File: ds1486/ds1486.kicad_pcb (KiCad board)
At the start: 4 copper layers, 30.4 x 43.9 mm, 76 parts, among them J1 DBG, J2 DBG1-16, J3 DBG17-32, J4 DS1-16, J5 DS17-32, U1 RP2040, U2 AP2112K-3.3, U3 W25Q16JVUXIQ, U4 SN74LVC8T245, U5 SN74LVC1G00DRL, U6 YSN8010SJ, U7 SN74LVC1G00DRL, Y2 E3SB12E00004EE

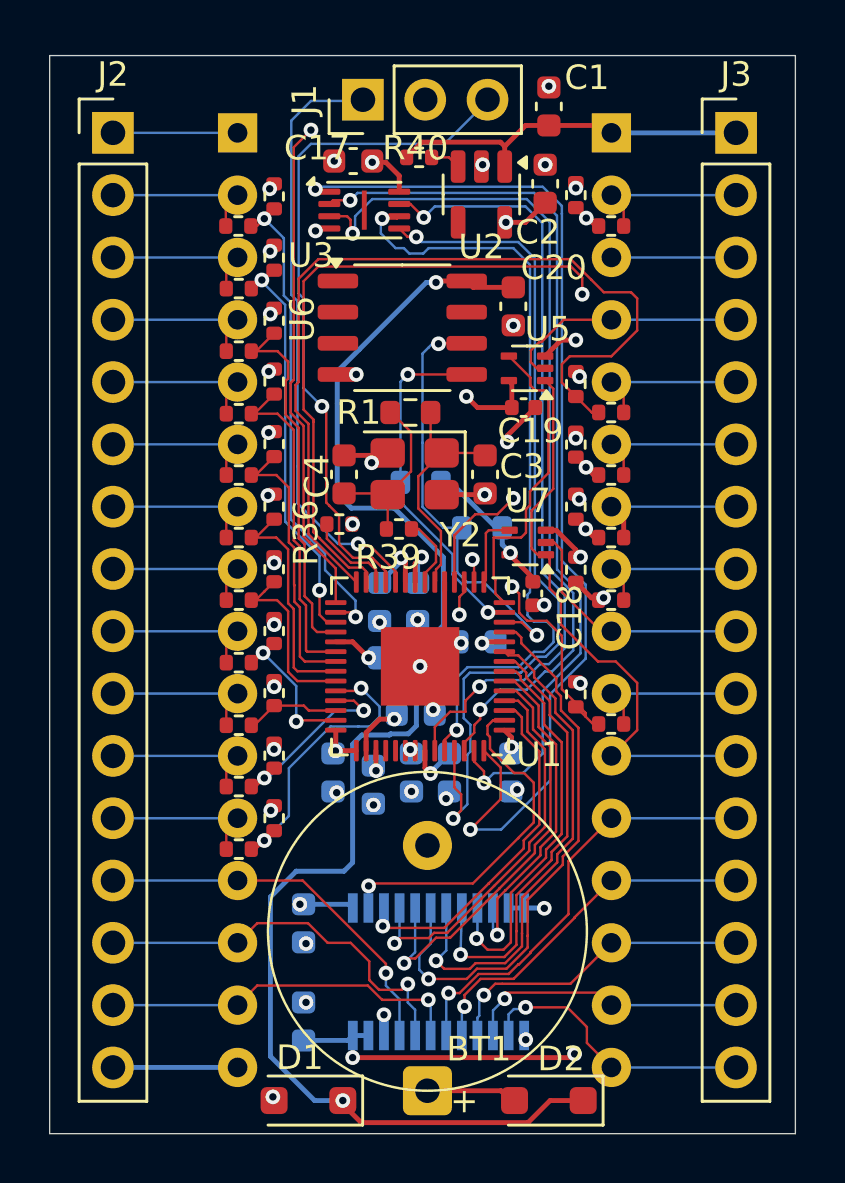
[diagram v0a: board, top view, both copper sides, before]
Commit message: Move D_DIR.
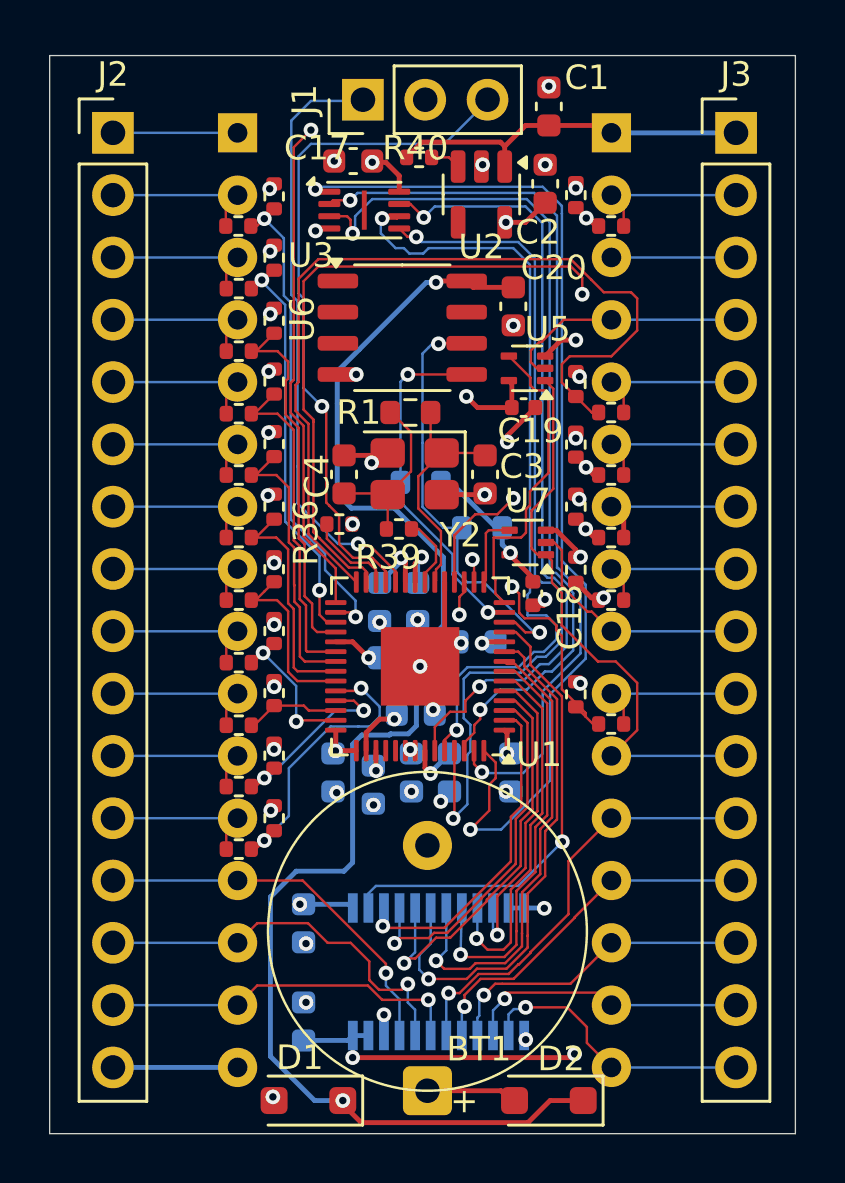
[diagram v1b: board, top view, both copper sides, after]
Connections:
- U1 pad 11: /DQC7 -> /D_DIR
- U1 pad 2: /D_DIR -> /DQC0
- U1 pad 3: /DQC0 -> /DQC1
- U1 pad 4: /DQC1 -> /DQC2
- U1 pad 5: /DQC2 -> /DQC3
- U1 pad 6: /DQC3 -> /DQC4
- U1 pad 7: /DQC4 -> /DQC5
- U1 pad 8: /DQC5 -> /DQC6
- U1 pad 9: /DQC6 -> /DQC7
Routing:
- net /D_DIR: track 14.5 -> 19.2 mm
- net /DQC3: track 14.5 -> 12.6 mm
- net /DQC7: track 23.1 -> 21.6 mm
- net /DQC6: track 20.6 -> 19.5 mm
- net /DQC5: track 18.5 -> 17.5 mm
- net /DQC1: track 16.0 -> 14.9 mm
- net /DQC2: track 17.6 -> 16.5 mm
- net /DQC0: track 14.6 -> 13.6 mm
- net GND: track 30.8 -> 31.5 mm
- net /DQC4: track 15.7 -> 15.1 mm
- net /QSPI_SD1: track 37.2 -> 36.7 mm
